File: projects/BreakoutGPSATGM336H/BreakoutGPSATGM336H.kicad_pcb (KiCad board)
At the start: 2 copper layers, 35.6 x 25.4 mm, 3 parts, among them J1 Conn_01x09_Female, J2 Conn_01x09_Female, U1 UBLOX_MAX-7

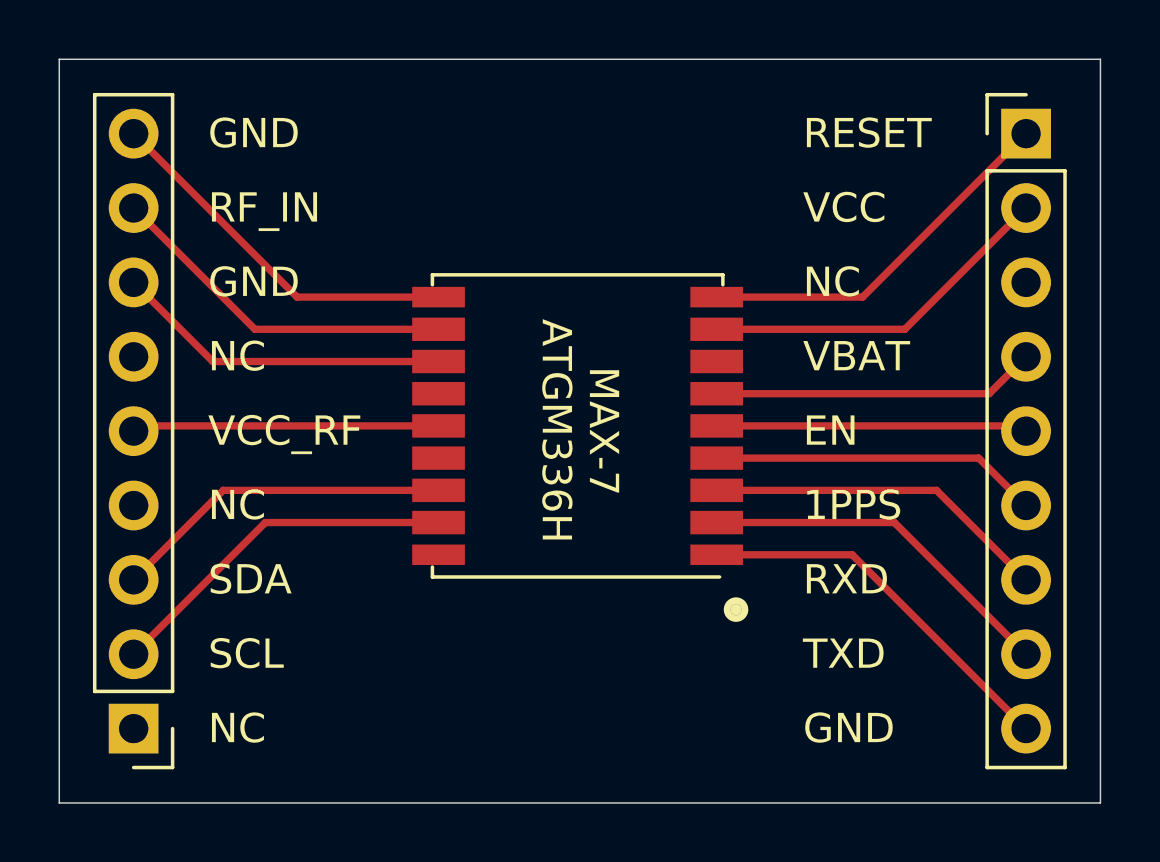
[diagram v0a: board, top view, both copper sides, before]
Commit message: BreakoutGPSATGM336H
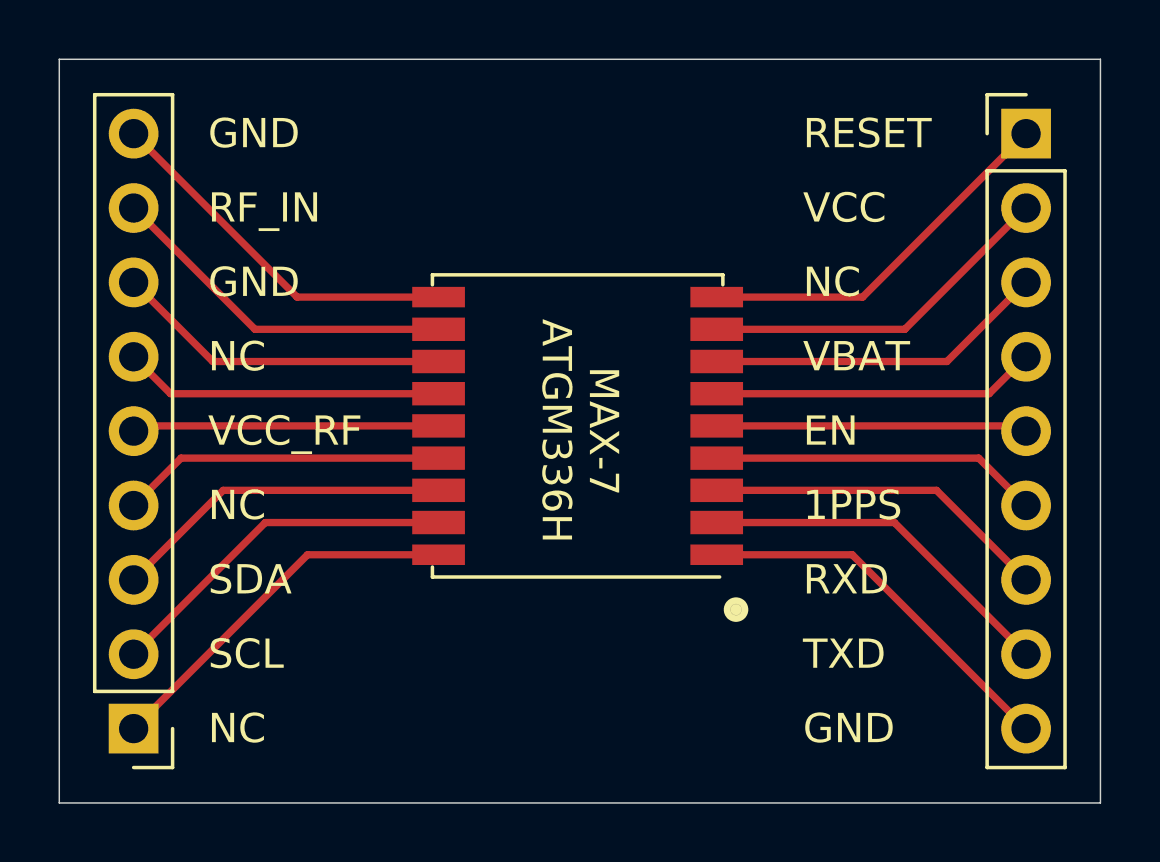
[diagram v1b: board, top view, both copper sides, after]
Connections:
- J1 pad 1: (no net) -> Net-(J1-Pad1)
- J1 pad 4: (no net) -> Net-(J1-Pad4)
- J1 pad 6: (no net) -> Net-(J1-Pad6)
- J2 pad 3: (no net) -> Net-(J2-Pad3)
- U1 pad 13: (no net) -> Net-(J1-Pad6)
- U1 pad 15: (no net) -> Net-(J1-Pad4)
- U1 pad 18: (no net) -> Net-(J1-Pad1)
- U1 pad 7: (no net) -> Net-(J2-Pad3)
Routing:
- net Net-(J1-Pad1): track 0.00 -> 12.9 mm
- net Net-(J2-Pad3): track 0.00 -> 11.7 mm
- net Net-(J1-Pad4): track 0.00 -> 11.1 mm
- net Net-(J1-Pad6): track 0.00 -> 10.9 mm
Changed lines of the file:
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@@
     (thickness 1.6)
     (drawings 28)
-    (tracks 28)
+    (tracks 36)
     (zones 0)
     (modules 3)
-    (nets 13)
+    (nets 17)
   )
   (page A4)
@@
     (solder_mask_min_width 0.25)
     (aux_axis_origin 0 0)
-    (visible_elements FFFFFF7F)
+    (visible_elements 7FFFFFFF)
     (pcbplotparams
       (layerselection 0x010fc_ffffffff)
@@
   (net 11 "Net-(J2-Pad1)")
   (net 12 GND)
+  (net 13 "Net-(J1-Pad1)")
+  (net 14 "Net-(J1-Pad4)")
+  (net 15 "Net-(J1-Pad6)")
+  (net 16 "Net-(J2-Pad3)")
   (net_class Default "This is the default net class."
     (clearance 0.2)
@@
     (uvia_drill 0.1)
     (add_net GND)
+    (add_net "Net-(J1-Pad1)")
     (add_net "Net-(J1-Pad2)")
     (add_net "Net-(J1-Pad3)")
+    (add_net "Net-(J1-Pad4)")
     (add_net "Net-(J1-Pad5)")
+    (add_net "Net-(J1-Pad6)")
     (add_net "Net-(J1-Pad8)")
     (add_net "Net-(J2-Pad1)")
     (add_net "Net-(J2-Pad2)")
+    (add_net "Net-(J2-Pad3)")
     (add_net "Net-(J2-Pad4)")
     (add_net "Net-(J2-Pad5)")
@@
       (effects (font (size 1 1) (thickness 0.15)))
     )
-    (pad 1 thru_hole rect (at 0 0 180) (size 1.7 1.7) (drill 1) (layers *.Cu *.Mask))
+    (pad 1 thru_hole rect (at 0 0 180) (size 1.7 1.7) (drill 1) (layers *.Cu *.Mask)
+      (net 13 "Net-(J1-Pad1)"))
     (pad 2 thru_hole oval (at 0 2.54 180) (size 1.7 1.7) (drill 1) (layers *.Cu *.Mask)
       (net 1 "Net-(J1-Pad2)"))
     (pad 3 thru_hole oval (at 0 5.08 180) (size 1.7 1.7) (drill 1) (layers *.Cu *.Mask)
       (net 2 "Net-(J1-Pad3)"))
-    (pad 4 thru_hole oval (at 0 7.62 180) (size 1.7 1.7) (drill 1) (layers *.Cu *.Mask))
+    (pad 4 thru_hole oval (at 0 7.62 180) (size 1.7 1.7) (drill 1) (layers *.Cu *.Mask)
+      (net 14 "Net-(J1-Pad4)"))
     (pad 5 thru_hole oval (at 0 10.16 180) (size 1.7 1.7) (drill 1) (layers *.Cu *.Mask)
       (net 3 "Net-(J1-Pad5)"))
-    (pad 6 thru_hole oval (at 0 12.7 180) (size 1.7 1.7) (drill 1) (layers *.Cu *.Mask))
+    (pad 6 thru_hole oval (at 0 12.7 180) (size 1.7 1.7) (drill 1) (layers *.Cu *.Mask)
+      (net 15 "Net-(J1-Pad6)"))
     (pad 7 thru_hole oval (at 0 15.24 180) (size 1.7 1.7) (drill 1) (layers *.Cu *.Mask)
       (net 12 GND))
@@
     (pad 4 thru_hole oval (at 0 7.62) (size 1.7 1.7) (drill 1) (layers *.Cu *.Mask)
       (net 9 "Net-(J2-Pad4)"))
-    (pad 3 thru_hole oval (at 0 5.08) (size 1.7 1.7) (drill 1) (layers *.Cu *.Mask))
+    (pad 3 thru_hole oval (at 0 5.08) (size 1.7 1.7) (drill 1) (layers *.Cu *.Mask)
+      (net 16 "Net-(J2-Pad3)"))
     (pad 2 thru_hole oval (at 0 2.54) (size 1.7 1.7) (drill 1) (layers *.Cu *.Mask)
       (net 10 "Net-(J2-Pad2)"))
@@
       (effects (font (size 1 1) (thickness 0.15)))
     )
-    (pad 18 smd rect (at -4.8262 4.2222 180) (size 1.8 0.7) (layers F.Cu F.Paste F.Mask))
+    (pad 18 smd rect (at -4.8262 4.2222 180) (size 1.8 0.7) (layers F.Cu F.Paste F.Mask)
+      (net 13 "Net-(J1-Pad1)"))
     (pad 17 smd rect (at -4.8262 3.1222 180) (size 1.8 0.8) (layers F.Cu F.Paste F.Mask)
       (net 1 "Net-(J1-Pad2)"))
     (pad 16 smd rect (at -4.8262 2.0222 180) (size 1.8 0.8) (layers F.Cu F.Paste F.Mask)
       (net 2 "Net-(J1-Pad3)"))
-    (pad 15 smd rect (at -4.8262 0.9222 180) (size 1.8 0.8) (layers F.Cu F.Paste F.Mask))
+    (pad 15 smd rect (at -4.8262 0.9222 180) (size 1.8 0.8) (layers F.Cu F.Paste F.Mask)
+      (net 14 "Net-(J1-Pad4)"))
     (pad 14 smd rect (at -4.8262 -0.1778 180) (size 1.8 0.8) (layers F.Cu F.Paste F.Mask)
       (net 3 "Net-(J1-Pad5)"))
-    (pad 13 smd rect (at -4.8262 -1.2778 180) (size 1.8 0.8) (layers F.Cu F.Paste F.Mask))
+    (pad 13 smd rect (at -4.8262 -1.2778 180) (size 1.8 0.8) (layers F.Cu F.Paste F.Mask)
+      (net 15 "Net-(J1-Pad6)"))
     (pad 12 smd rect (at -4.8262 -2.3778 180) (size 1.8 0.8) (layers F.Cu F.Paste F.Mask)
       (net 12 GND))
@@
     (pad 8 smd rect (at 4.6738 -3.4778 180) (size 1.8 0.8) (layers F.Cu F.Paste F.Mask)
       (net 10 "Net-(J2-Pad2)"))
-    (pad 7 smd rect (at 4.6738 -2.3778 180) (size 1.8 0.8) (layers F.Cu F.Paste F.Mask))
+    (pad 7 smd rect (at 4.6738 -2.3778 180) (size 1.8 0.8) (layers F.Cu F.Paste F.Mask)
+      (net 16 "Net-(J2-Pad3)"))
     (pad 6 smd rect (at 4.6738 -1.2778 180) (size 1.8 0.8) (layers F.Cu F.Paste F.Mask)
       (net 9 "Net-(J2-Pad4)"))
@@
   (segment (start 162.0578 76.7022) (end 167.64 71.12) (width 0.25) (layer F.Cu) (net 11) (status 20))
   (segment (start 157.0738 76.7022) (end 162.0578 76.7022) (width 0.25) (layer F.Cu) (net 11) (status 10))
-  (segment (start 142.7422 76.7022) (end 137.16 71.12) (width 0.25) (layer F.Cu) (net 12))
-  (segment (start 147.5738 76.7022) (end 142.7422 76.7022) (width 0.25) (layer F.Cu) (net 12))
-  (segment (start 139.8622 78.9022) (end 137.16 76.2) (width 0.25) (layer F.Cu) (net 12))
-  (segment (start 147.5738 78.9022) (end 139.8622 78.9022) (width 0.25) (layer F.Cu) (net 12))
-  (segment (start 157.0738 85.5022) (end 161.7022 85.5022) (width 0.25) (layer F.Cu) (net 12))
-  (segment (start 161.7022 85.5022) (end 167.64 91.44) (width 0.25) (layer F.Cu) (net 12))
+  (segment (start 142.7422 76.7022) (end 137.16 71.12) (width 0.25) (layer F.Cu) (net 12) (status 20))
+  (segment (start 147.5738 76.7022) (end 142.7422 76.7022) (width 0.25) (layer F.Cu) (net 12) (status 10))
+  (segment (start 139.8622 78.9022) (end 137.16 76.2) (width 0.25) (layer F.Cu) (net 12) (status 20))
+  (segment (start 147.5738 78.9022) (end 139.8622 78.9022) (width 0.25) (layer F.Cu) (net 12) (status 10))
+  (segment (start 157.0738 85.5022) (end 161.7022 85.5022) (width 0.25) (layer F.Cu) (net 12) (status 10))
+  (segment (start 161.7022 85.5022) (end 167.64 91.44) (width 0.25) (layer F.Cu) (net 12) (status 20))
+  (segment (start 143.0978 85.5022) (end 137.16 91.44) (width 0.25) (layer F.Cu) (net 13))
+  (segment (start 147.5738 85.5022) (end 143.0978 85.5022) (width 0.25) (layer F.Cu) (net 13))
+  (segment (start 138.7778 82.2022) (end 137.16 83.82) (width 0.25) (layer F.Cu) (net 14))
+  (segment (start 147.5738 82.2022) (end 138.7778 82.2022) (width 0.25) (layer F.Cu) (net 14))
+  (segment (start 138.4222 80.0022) (end 137.16 78.74) (width 0.25) (layer F.Cu) (net 15))
+  (segment (start 147.5738 80.0022) (end 138.4222 80.0022) (width 0.25) (layer F.Cu) (net 15))
+  (segment (start 164.9378 78.9022) (end 167.64 76.2) (width 0.25) (layer F.Cu) (net 16))
+  (segment (start 157.0738 78.9022) (end 164.9378 78.9022) (width 0.25) (layer F.Cu) (net 16))
 )
